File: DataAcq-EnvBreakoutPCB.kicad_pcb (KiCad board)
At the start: 2 copper layers, 19.4 x 27.2 mm, 20 parts, among them J4 Breakout Connector, U1 FS3000-1005, U2 LMT87DCK, U3 SHT45

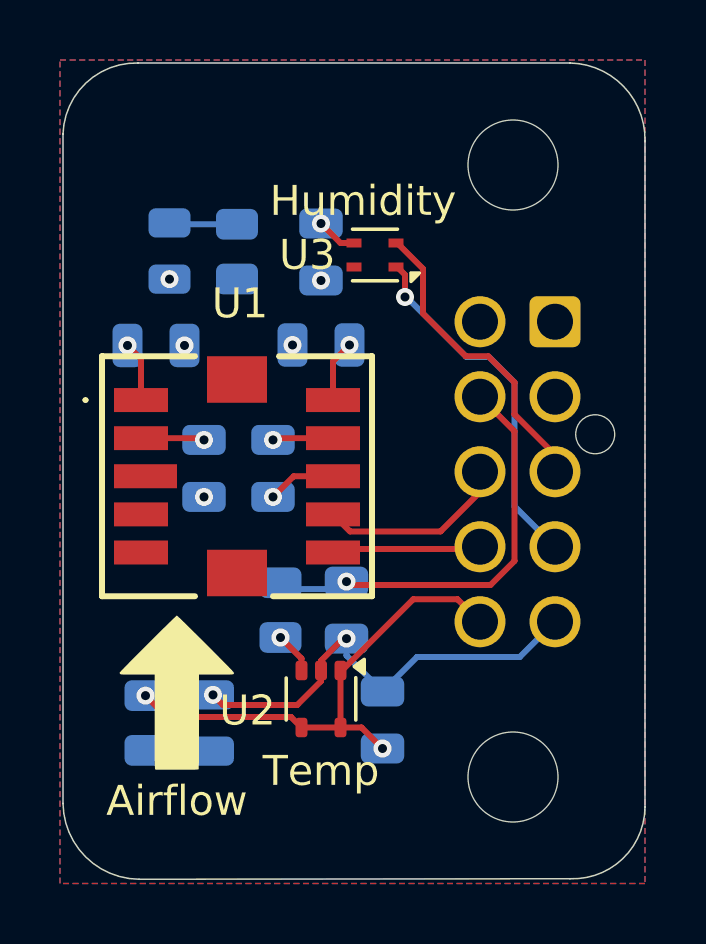
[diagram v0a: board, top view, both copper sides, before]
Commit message: better routing
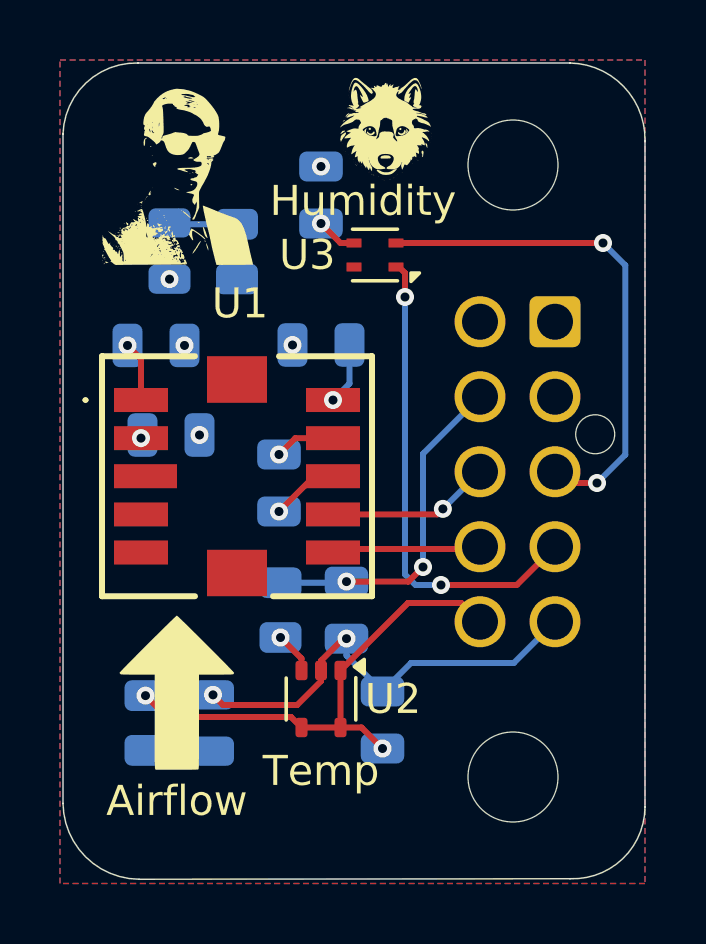
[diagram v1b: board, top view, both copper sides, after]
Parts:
- added G***: LOGO, LOGO, F.Cu at (122.8, 32.2)
- added G***: LOGO, LOGO, F.Cu at (115.8, 33.8)
- moved LOGO3 2.24 mm to (115.0, 46.8), turned to 180 degrees
- moved C7 1.90 mm to (120.6, 34.4), turned to 90 degrees
- moved C1 1.57 mm to (115.6, 42.4), turned to 0 degrees
- moved C4 0.52 mm to (119.2, 44.0)
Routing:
- net /I2C1_SCL: track 10.3 -> 17.2 mm, vias 0 -> 2
- net /I2C1_SDA: track 12.0 -> 16.1 mm, vias 1 -> 2
- net /PA1(ADC): track 14.2 -> 11.4 mm, vias 1 -> 2
- net +3.3V: track 3.49 -> 1.37 mm
- net /I2C2_SCL: track 6.36 -> 5.49 mm, vias 0 -> 1
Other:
- board text added: "MainConn"
